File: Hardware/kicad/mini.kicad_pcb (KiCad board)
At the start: 2 copper layers, 33 parts, among them J1 JS40F-I, J10 MOTOR-I, J11 MOTOR-D, J13 XT30PW-M, J2 JS40F-LI, J3 QRE-I, J4 JS40F-M, J5 QRE-M, J6 JS40F-D, J7 JS40F-LD, J8 QRE-D, SW2 SW_Push, SW4 SW_DIP_x03, U1 L7805, U2 TA6586, U3 ESP32-C3_SUPERMINI_TH, U4 TA6586

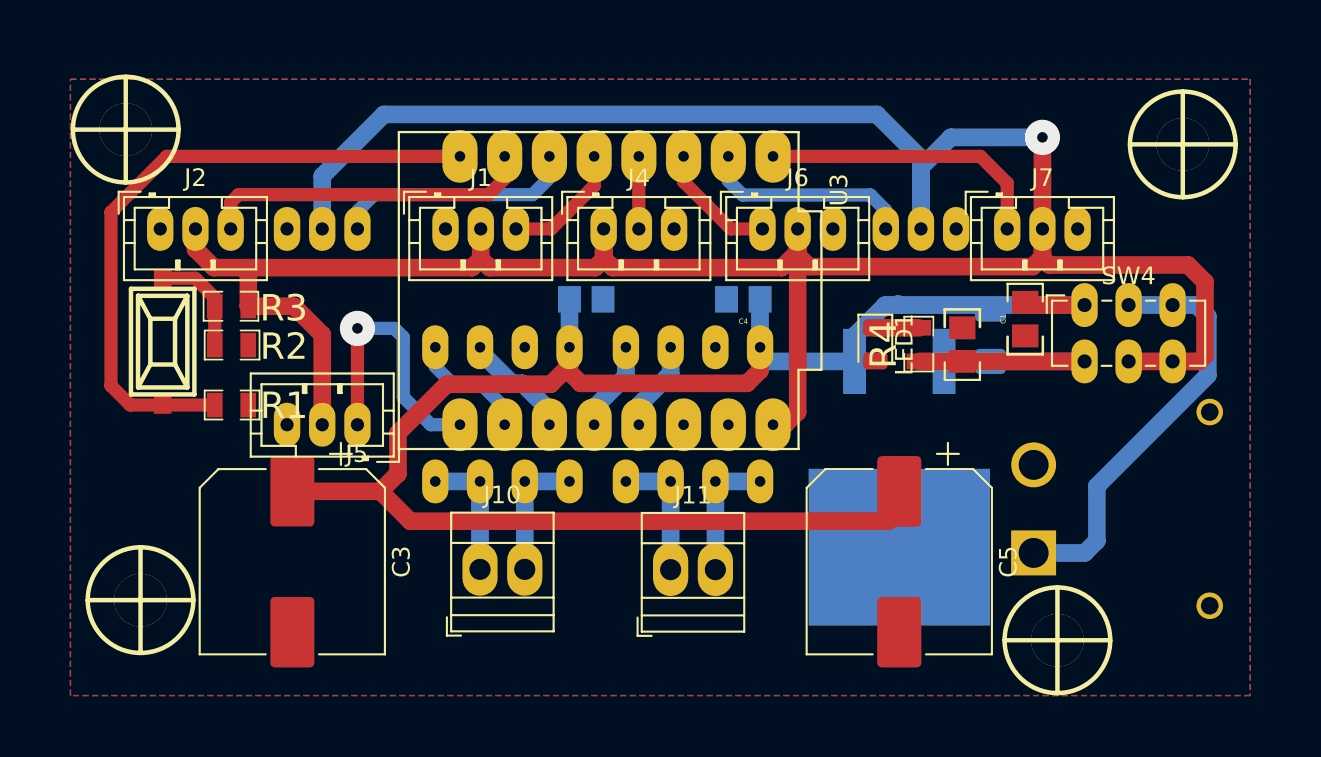
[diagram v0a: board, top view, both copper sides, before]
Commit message: actu 29/05
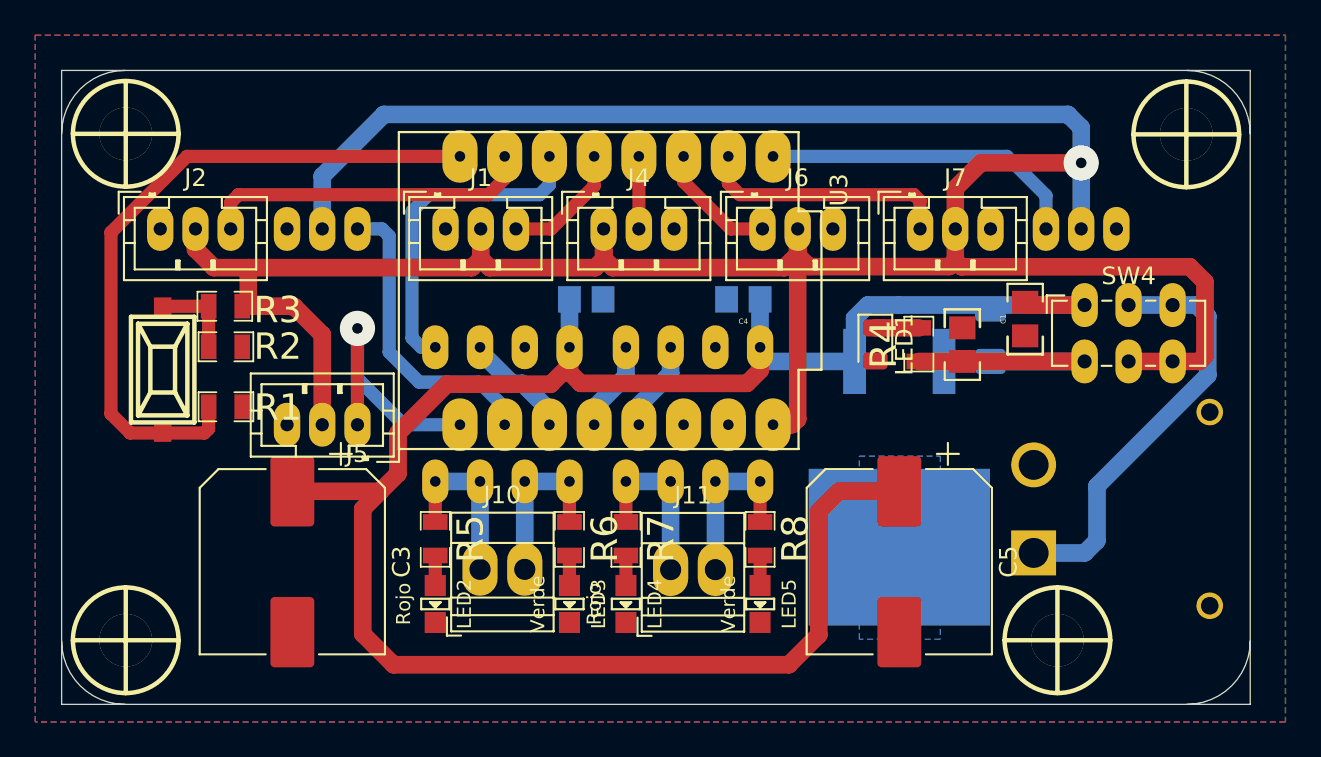
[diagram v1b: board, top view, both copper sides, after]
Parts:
- removed hole_3mm (x4): VAL**, EESTN5:hole_3mm
- added H1: Mounting_Hole, EESTN5:hole_3mm, F.Cu at (82.1, 37.1)
- added H2: Mounting_Hole, EESTN5:hole_3mm, F.Cu at (82.1, 65.9)
- added H3: Mounting_Hole, EESTN5:hole_3mm, F.Cu at (142.4, 37.1)
- added H4: Mounting_Hole, EESTN5:hole_3mm, F.Cu at (135.1, 65.9)
- added LED2: Rojo, EESTN5:Led_0805, F.Cu at (99.7, 63.8)
- added LED3: Verde, EESTN5:Led_0805, F.Cu at (107.3, 63.8)
- added LED4: Rojo, EESTN5:Led_0805, F.Cu at (110.5, 63.8)
- added LED5: Verde, EESTN5:Led_0805, F.Cu at (118.2, 63.8)
- added R5: 22k, EESTN5:R_0805, F.Cu at (99.7, 60.1)
- added R6: 22k, EESTN5:R_0805, F.Cu at (107.3, 60.1)
- added R7: 22k, EESTN5:R_0805, F.Cu at (110.5, 60.1)
- added R8: 22k, EESTN5:R_0805, F.Cu at (118.2, 60.1)
- moved J8 9.10 mm to (138.4, 42.5)
- moved J7 4.95 mm to (127.2, 42.5)
- moved SW2 1.59 mm to (84.2, 50.5)
- moved R1 0.36 mm to (87.8, 52.6)
- moved R3 0.36 mm to (87.8, 49.2)
- moved R2 0.35 mm to (87.8, 46.9)
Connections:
- U3 pad 1: /MI_A -> /QRE-I
- U3 pad 10: /QRE-I -> /MI_A
- U3 pad 5: /JS40F-LD -> /QRE-D
- U3 pad 6: /QRE-D -> /JS40F-LD
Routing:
- net VCC: track 96.6 -> 113.5 mm
- net /MI_A: track 6.97 -> 18.8 mm
- net /QRE-D: track 12.1 -> 18.3 mm
- net /QRE-I: track 13.9 -> 17.4 mm
- net +5V: track 163.8 -> 166.4 mm
- net Net-(U4-FO1): track 7.55 -> 9.86 mm
- net Net-(U4-BO1): track 7.55 -> 9.86 mm
- net Net-(U2-FO1): track 7.53 -> 9.84 mm
- net Net-(U2-BO1): track 7.53 -> 9.84 mm
- net /JS40F-LD: track 16.5 -> 14.4 mm
- net /START: track 37.3 -> 39.3 mm
- net Net-(LED5-A): track 0.00 -> 1.70 mm
- net Net-(LED4-A): track 0.00 -> 1.70 mm
- net Net-(LED3-A): track 0.00 -> 1.70 mm
- net Net-(LED2-A): track 0.00 -> 1.70 mm
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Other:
- board outline added: 67.5 x 36 mm
